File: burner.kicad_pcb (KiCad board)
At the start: 2 copper layers, 118.8 x 58.4 mm, 76 parts, among them IC1 MAX6675, IC2 MAX6675, J1 MCU_ISP, J12 USB_A, J13 FTDI, J14 ENCODER, J2 220V_INPUT, J3 5V_INPUT, J4 BURNER2, J5 BURNER1, J6 1604_conn, J7 I2C_DISPLAY, J8 KTYPE1, J9 KTYPE1, Q1 AOD417, U1 ATmega2560-16AU, U2 4N25, U3 4N25, U4 ULN2003A, U5 AZ943, U6 AZ943, U7 CP2102N-A01-GQFN28, Y1 16MHz

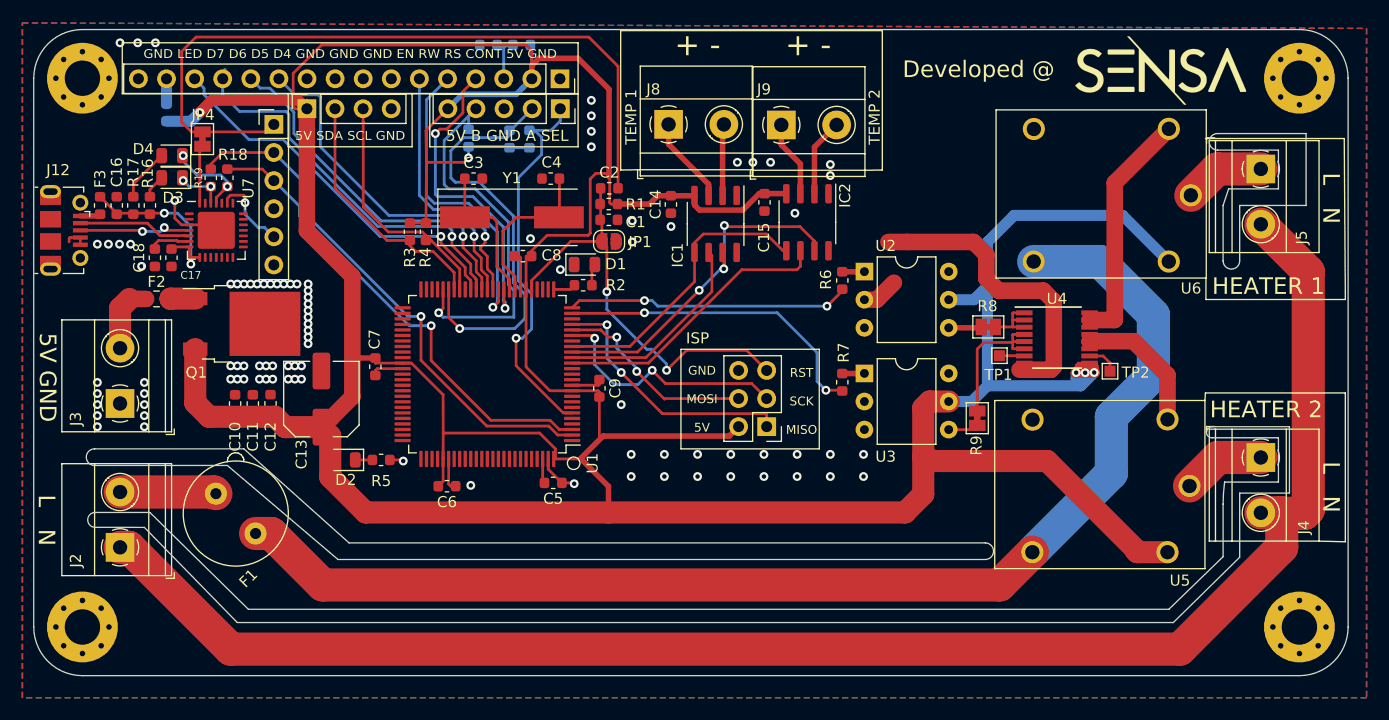
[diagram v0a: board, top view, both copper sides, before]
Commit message: update
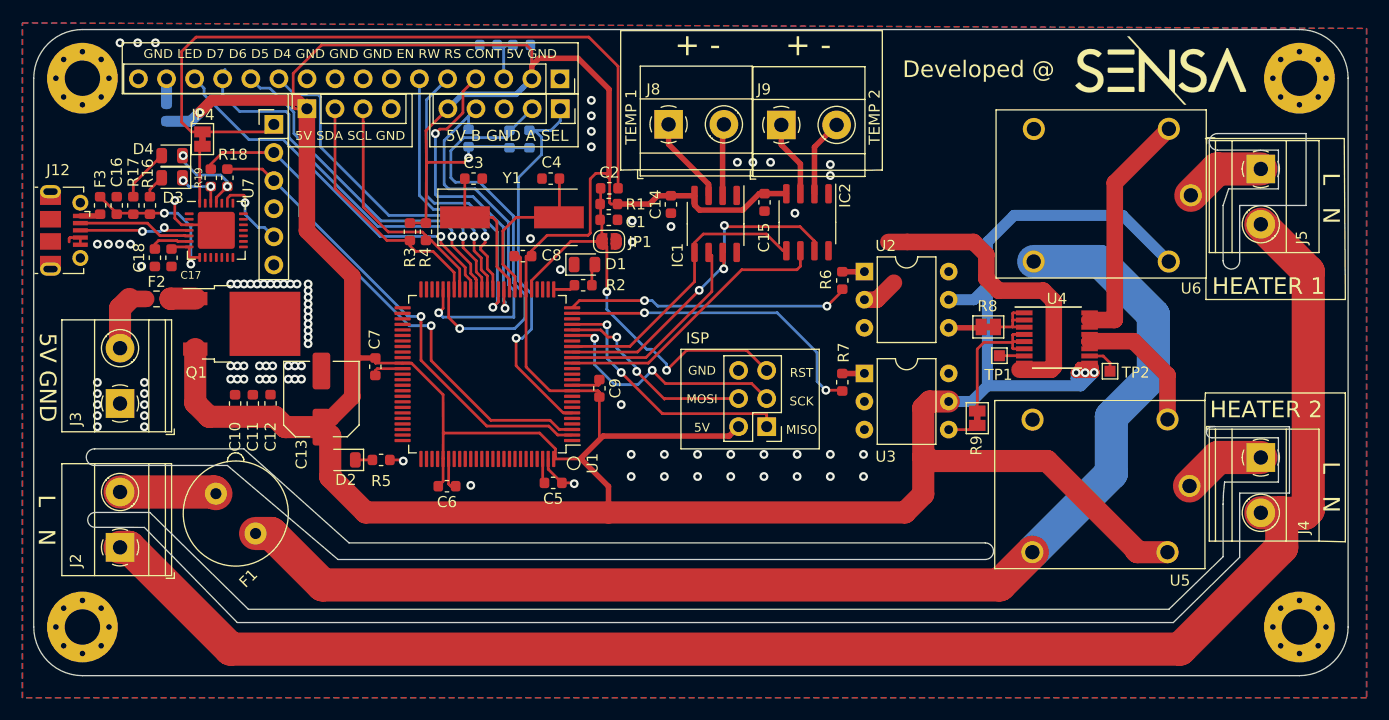
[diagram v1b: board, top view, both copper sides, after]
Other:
- net class Default removed
